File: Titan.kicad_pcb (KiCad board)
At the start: 4 copper layers, 60 x 115 mm, 155 parts, among them J1 USB_B_Micro, J10 PWM1, J11 SPI SLAVE, J12 IO Conn 2, J13 IO Conn 1, J14 ADC EXT, J15 PWM2, J2 USB_B_Micro, J3 Uart 1, J4 Bat Conn, J5 Debug, J6 Uart 2, J7 SPI AUX MASTER, J8 S3B-ZR(LF)(SN), J9 S3B-ZR(LF)(SN), Q1 NDS332P, Q2 NDS332P, SW1 SW_Push, SW2 SW_DPDT_x2, U1 FT230XS, U2 SR10S3V3, U3 STM32F413VGTx, U4 CY15B104Q, U5 MPU-6050, U6 FT230XS, U7 XBEE3Micro, U8 MPU-6050

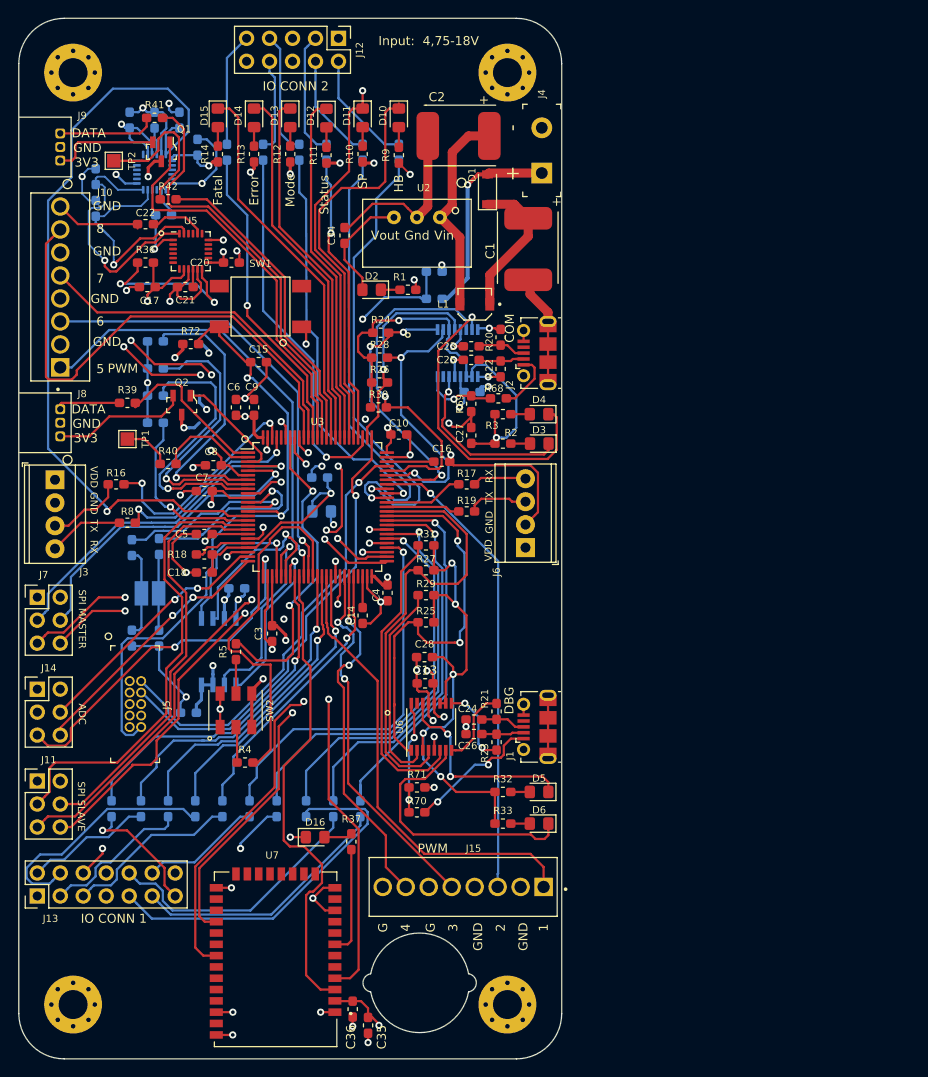
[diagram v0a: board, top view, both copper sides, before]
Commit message: First commit of TitanV2
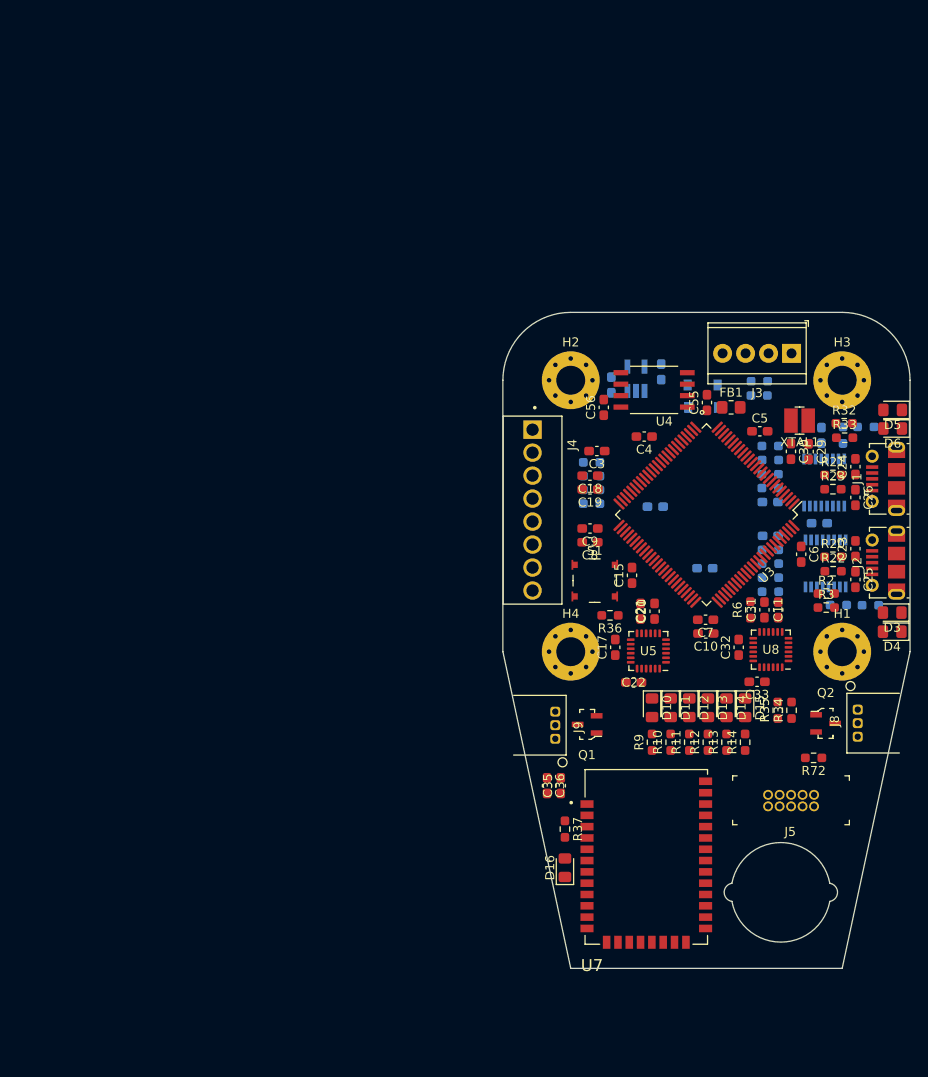
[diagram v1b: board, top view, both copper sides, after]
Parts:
- removed C2: 470uF, Titan:T59EE477M016C0025
- removed J10: PWM1, Footprint:HDRV8W85P254_8X1_2078X650X1000
- removed J11: SPI SLAVE, Connector_PinHeader_2.54mm:PinHeader_2x03_P2.54mm_Vertical
- removed J12: IO Conn 2, Connector_PinHeader_2.54mm:PinHeader_2x05_P2.54mm_Vertical
- removed J13: IO Conn 1, Connector_PinHeader_2.54mm:PinHeader_2x07_P2.54mm_Vertical
- removed J14: ADC EXT, Connector_PinHeader_2.54mm:PinHeader_2x03_P2.54mm_Vertical
- removed J15: PWM2, Footprint:HDRV8W85P254_8X1_2078X650X1000
- removed J6: Uart 2, TerminalBlock_TE-Connectivity:TerminalBlock_TE_282834-4_1x04_P2.54mm_Horizontal
- removed J7: SPI AUX MASTER, Connector_PinHeader_2.54mm:PinHeader_2x03_P2.54mm_Vertical
- removed L1: 1231AS-H-6R4M=P3, Footprint:IND_1231AS-H-6R4M=P3
- removed R1: 330, Resistor_SMD:R_0603_1608Metric_Pad1.05x0.95mm_HandSolder
- removed R16, R17, R19, R39, R40, R41, R42, R8: 220, Resistor_SMD:R_0603_1608Metric_Pad1.05x0.95mm_HandSolder
- removed R18, R63, R7: 0, Resistor_SMD:R_0603_1608Metric_Pad1.05x0.95mm_HandSolder
- removed R4, R5: 10k, Resistor_SMD:R_0603_1608Metric_Pad1.05x0.95mm_HandSolder
- removed R43, R44, R45, R46, R47, R48, R49, R50, R51, R52, R53, R54, R55, R56, R57, R58: 1K, Resistor_SMD:R_0603_1608Metric_Pad1.05x0.95mm_HandSolder
- removed SW1: SW_Push, Titan:TL3301AF160QG
- removed SW2: SW_DPDT_x2, Titan:CASD20
- removed TP1, TP2: TestPoint, TestPoint:TestPoint_Pad_1.5x1.5mm
- added S1: Reset button, digikey-footprints:Switch_Tactile_SMD_4.5x4.5mm_TL3315NF160Q, F.Cu at (127.7, 92.1)
- C1: value 470uF -> 2.2uF; footprint Titan:T59EE477M016C0025 -> Capacitor_SMD:C_0603_1608Metric_Pad1.08x0.95mm_HandSolder; moved to B.Cu
- C10, C12, C15, C17, C18, C20, C21, C22, C23, C24, C25, C26, C3, C35, C36, C4, C5, C6, C7, C8, C9: footprint Capacitor_SMD:C_0603_1608Metric_Pad1.05x0.95mm_HandSolder -> Capacitor_SMD:C_0603_1608Metric_Pad1.08x0.95mm_HandSolder
- C11, C19, C29, C30, C31, C32, C33, C55, C56: footprint Capacitor_SMD:C_0603_1608Metric_Pad1.05x0.95mm_HandSolder -> Capacitor_SMD:C_0603_1608Metric_Pad1.08x0.95mm_HandSolder; moved to F.Cu
- C13, C14, C16, C27, C28: footprint Capacitor_SMD:C_0603_1608Metric_Pad1.05x0.95mm_HandSolder -> Capacitor_SMD:C_0603_1608Metric_Pad1.08x0.95mm_HandSolder; moved to B.Cu
- C34: value 22uF -> 2.2uF; footprint Capacitor_SMD:C_0603_1608Metric_Pad1.05x0.95mm_HandSolder -> Capacitor_SMD:C_0603_1608Metric_Pad1.08x0.95mm_HandSolder; moved to B.Cu
- D1, U6: moved to B.Cu
- D2: value PWR_ON -> D_Schottky; footprint LED_SMD:LED_0805_2012Metric_Pad1.15x1.40mm_HandSolder -> Diode_SMD:D_SOD-123; moved to B.Cu
- FB1: footprint Resistor_SMD:R_0805_2012Metric_Pad1.15x1.40mm_HandSolder -> Resistor_SMD:R_0805_2012Metric_Pad1.20x1.40mm_HandSolder; moved to F.Cu
- J3: value Uart 1 -> PWR CON
- J4: value Bat Conn -> Screw_Terminal_01x08; footprint digikey-footprints:Terminal_Block_D1.3mm_P5mm -> Footprint:HDRV8W85P254_8X1_2078X650X1000
- Q1, Q2: footprint digikey-footprints:SOT-23-3 -> Titan:SOT-23-3
- R10, R11, R12, R13, R14, R15, R2, R20, R21, R22, R23, R3, R32, R33, R36, R37, R38, R59, R60, R61, R62, R72, R9: footprint Resistor_SMD:R_0603_1608Metric_Pad1.05x0.95mm_HandSolder -> Resistor_SMD:R_0603_1608Metric_Pad0.98x0.95mm_HandSolder
- R24, R25, R26, R27, R28, R29, R30, R31, R68, R69, R70, R71: footprint Resistor_SMD:R_0603_1608Metric_Pad1.05x0.95mm_HandSolder -> Resistor_SMD:R_0603_1608Metric_Pad0.98x0.95mm_HandSolder; moved to B.Cu
- R34, R35, R6: footprint Resistor_SMD:R_0603_1608Metric_Pad1.05x0.95mm_HandSolder -> Resistor_SMD:R_0603_1608Metric_Pad0.98x0.95mm_HandSolder; moved to F.Cu
- U2: value SR10S3V3 -> ST730M33R; footprint Titan:SR10S3V3 -> Package_TO_SOT_SMD:SOT-23-5_HandSoldering; moved to B.Cu
- U4, U8, XTAL1: moved to F.Cu
- moved R34 96.9 mm to (149.4, 106.5), turned to 90 degrees
- moved R35 93.6 mm to (147.9, 106.5), turned to 90 degrees
- moved H1 93.5 mm to (155.0, 100.0)
- moved J8 93.2 mm to (156.7, 106.4), turned to 270 degrees
- moved C11 89.8 mm to (147.9, 95.4)
- moved D15 87.4 mm to (144.3, 106.2)
- moved R14 87.3 mm to (144.3, 110.0)
- moved C31 86.4 mm to (146.4, 95.4)
- moved U8 86.2 mm to (147.1, 99.8), turned to 180 degrees
- moved H4 84.4 mm to (125.0, 100.0)
- moved J9 84.1 mm to (123.3, 109.6)
- moved D14 83.5 mm to (142.2, 106.2)
- moved C33 83.4 mm to (145.6, 103.3)
- moved R13 83.4 mm to (142.2, 110.0)
- moved R6 83.1 mm to (144.9, 95.4)
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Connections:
- D2 pad 1: Net-(D2-Pad1) -> Net-(C1-Pad1)
- D2 pad 2: VDD_MCU -> /VBUS_COM
- J1 pad 1: Net-(J1-Pad1) -> /VBUS_COM
- J3 pad 1: VDD_MCU -> GND
- J3 pad 2: GND -> VDD_MCU
- J3 pad 3: Net-(J3-Pad3) -> GND
- J3 pad 4: Net-(J3-Pad4) -> Net-(D1-Pad2)
- J4 pad 1: Net-(D1-Pad2) -> /PWM_1
- J4 pad 2: GND -> /PWM_2
- J8 pad 3: Net-(J8-Pad3) -> /UART_RC_1_RX
- J9 pad 3: Net-(J9-Pad3) -> /UART_RC_2_RX
- R59 pad 1: GND -> VDD_MCU
- R70 pad 1: Net-(J1-Pad1) -> /VBUS_COM
- U2 pad 1: Net-(C2-Pad1) -> VDD_MCU
- U2 pad 3: VDD_MCU -> Net-(C1-Pad1)
- U3 pad 12: Net-(R7-Pad1) -> Net-(C29-Pad1)
- U3 pad 13: Net-(R63-Pad1) -> Net-(C30-Pad1)
- U3 pad 17: SPI_SLAVE_MISO -> (no net)
- U3 pad 18: SPI_SLAVE_MOSI -> (no net)
- U3 pad 2: /UART_RC_1_TX -> (no net)
- U3 pad 21: Net-(R18-Pad1) -> VDDA_MCU
- U3 pad 24: ADC_1 -> (no net)
- U3 pad 25: ADC_2 -> (no net)
- U3 pad 26: ADC_3 -> (no net)
- U3 pad 33: /IO_12 -> (no net)
- U3 pad 35: /PWM_5 -> (no net)
- U3 pad 36: /PWM_6 -> (no net)
- U3 pad 37: BOOT1 -> (no net)
- U3 pad 38: /IO_1 -> (no net)
- U3 pad 39: /IO_2 -> (no net)
- U3 pad 4: SPI_AUX_MISO -> (no net)
- U3 pad 41: /IO_3 -> (no net)
- U3 pad 42: SPI_AUX_NSS -> (no net)
- U3 pad 43: SPI_AUX_SCK -> (no net)
- U3 pad 46: /IO_4 -> (no net)
- U3 pad 5: SPI_AUX_MOSI -> (no net)
- U3 pad 51: SPI_SLAVE_NSS -> (no net)
- U3 pad 52: SPI_SLAVE_SCK -> (no net)
- U3 pad 54: /IO_11 -> (no net)
- U3 pad 56: /IO_5 -> (no net)
- U3 pad 57: /IO_6 -> (no net)
- U3 pad 59: /IO_7 -> (no net)
- U3 pad 60: /IO_8 -> (no net)
- U3 pad 65: /IO_13 -> (no net)
- U3 pad 66: /IO_14 -> (no net)
- U3 pad 67: /IO_9 -> (no net)
- U3 pad 78: /IO_15 -> (no net)
- U3 pad 79: /IO_10 -> (no net)
- U3 pad 86: /UART_RC_2_TX -> (no net)
- U3 pad 89: /IO_16 -> (no net)
- U3 pad 90: /PWM_7 -> (no net)
- U3 pad 91: /PWM_8 -> (no net)
- U3 pad 94: BOOT0 -> GND
- U3 pad 97: /UART_MOTOR_1_RX -> (no net)
- U3 pad 98: /UART_MOTOR_1_TX -> (no net)
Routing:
- net GND: track 253.7 -> 0.00 mm, vias 44 -> 0
- net VDD_MCU: track 139.1 -> 0.00 mm, vias 31 -> 0
- net /IMU2_INT: track 88.5 -> 0.00 mm, vias 1 -> 0
- net /nRESET: track 72.8 -> 0.00 mm, vias 2 -> 0
- net /I2C_SDA_IMU: track 69.1 -> 0.00 mm, vias 4 -> 0
- net /I2C_SCL_IMU: track 61.1 -> 0.00 mm, vias 4 -> 0
- net Net-(C28-Pad2): track 59.6 -> 0.00 mm, vias 5 -> 0
- net /UART_COM_CTS: track 59.4 -> 0.00 mm, vias 2 -> 0
- net /PWM_8: track 57.5 -> 0.00 mm
- net SPI_SLAVE_NSS: track 56.2 -> 0.00 mm, vias 2 -> 0
- net /UART_COM_TX: track 55.3 -> 0.00 mm, vias 2 -> 0
- net SPI_SLAVE_SCK: track 54.1 -> 0.00 mm, vias 2 -> 0
- net /UART_COM_RX: track 53.3 -> 0.00 mm
- net /UART_COM_RTS: track 53.2 -> 0.00 mm, vias 2 -> 0
- net /ADC_BAT: track 53.0 -> 0.00 mm, vias 5 -> 0
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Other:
- board size 60 x 115 mm -> 45 x 72.5 mm
- board text removed: "+"
- board text removed: "-"
- board text removed: "1"
- board text removed: "2"
- board text removed: "3"
- board text removed: "4"
- board text removed: "5"
- board text removed: "6"
- board text removed: "7"
- board text removed: "8"
- board text removed: "ADC"
- board text removed: "COM"
- board text removed: "DBG"
- board text removed: "Error"
- board text removed: "Fatal"
- board text removed: "G"
- board text removed: "GND"
- board text removed: "HB"
- board text removed: "IO CONN 1"
- board text removed: "IO CONN 2"
- board text removed: "Input: 4,75-18V"
- board text removed: "Mode"
- board text removed: "PWM"
- board text removed: "RX"
- board text removed: "SP"
- board text removed: "SPI MASTER"
- board text removed: "SPI SLAVE"
- board text removed: "Status"
- board text removed: "TX"
- board text removed: "Titan V1.0"
- board text removed: "VDD"
